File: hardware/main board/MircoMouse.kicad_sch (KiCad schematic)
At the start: 43 parts, among them IC4 W25N01GVZEIG, IC5 LSM6DSLTR, J1 JST-SH 01x06, J2 JST-SH 01x06, J3 JST_XH_B3B, J4 FTSH-107-01-L-DV-K-A, J5 JST-SH 01x06, J6 USB4145-03-0070-C, J7 JST-SH 01x06, U1 LM1117MP-3.3, U2 USBLC6-2SC6

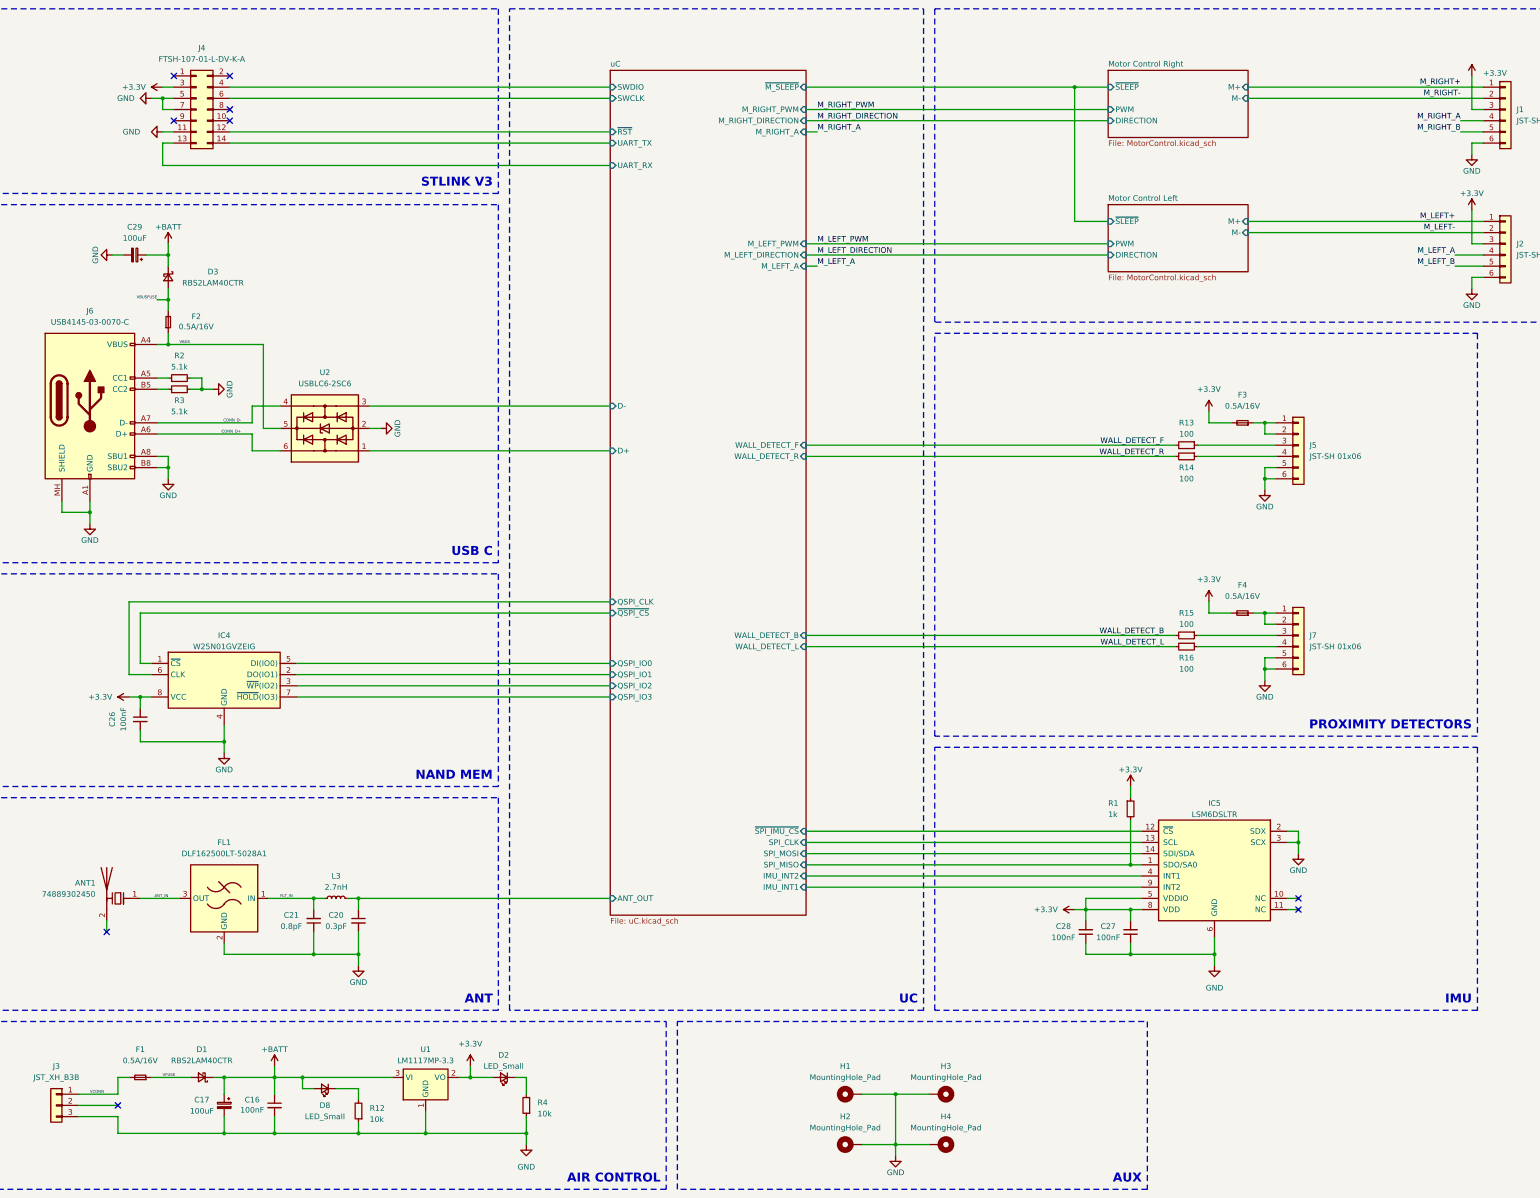
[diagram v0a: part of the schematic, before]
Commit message: final
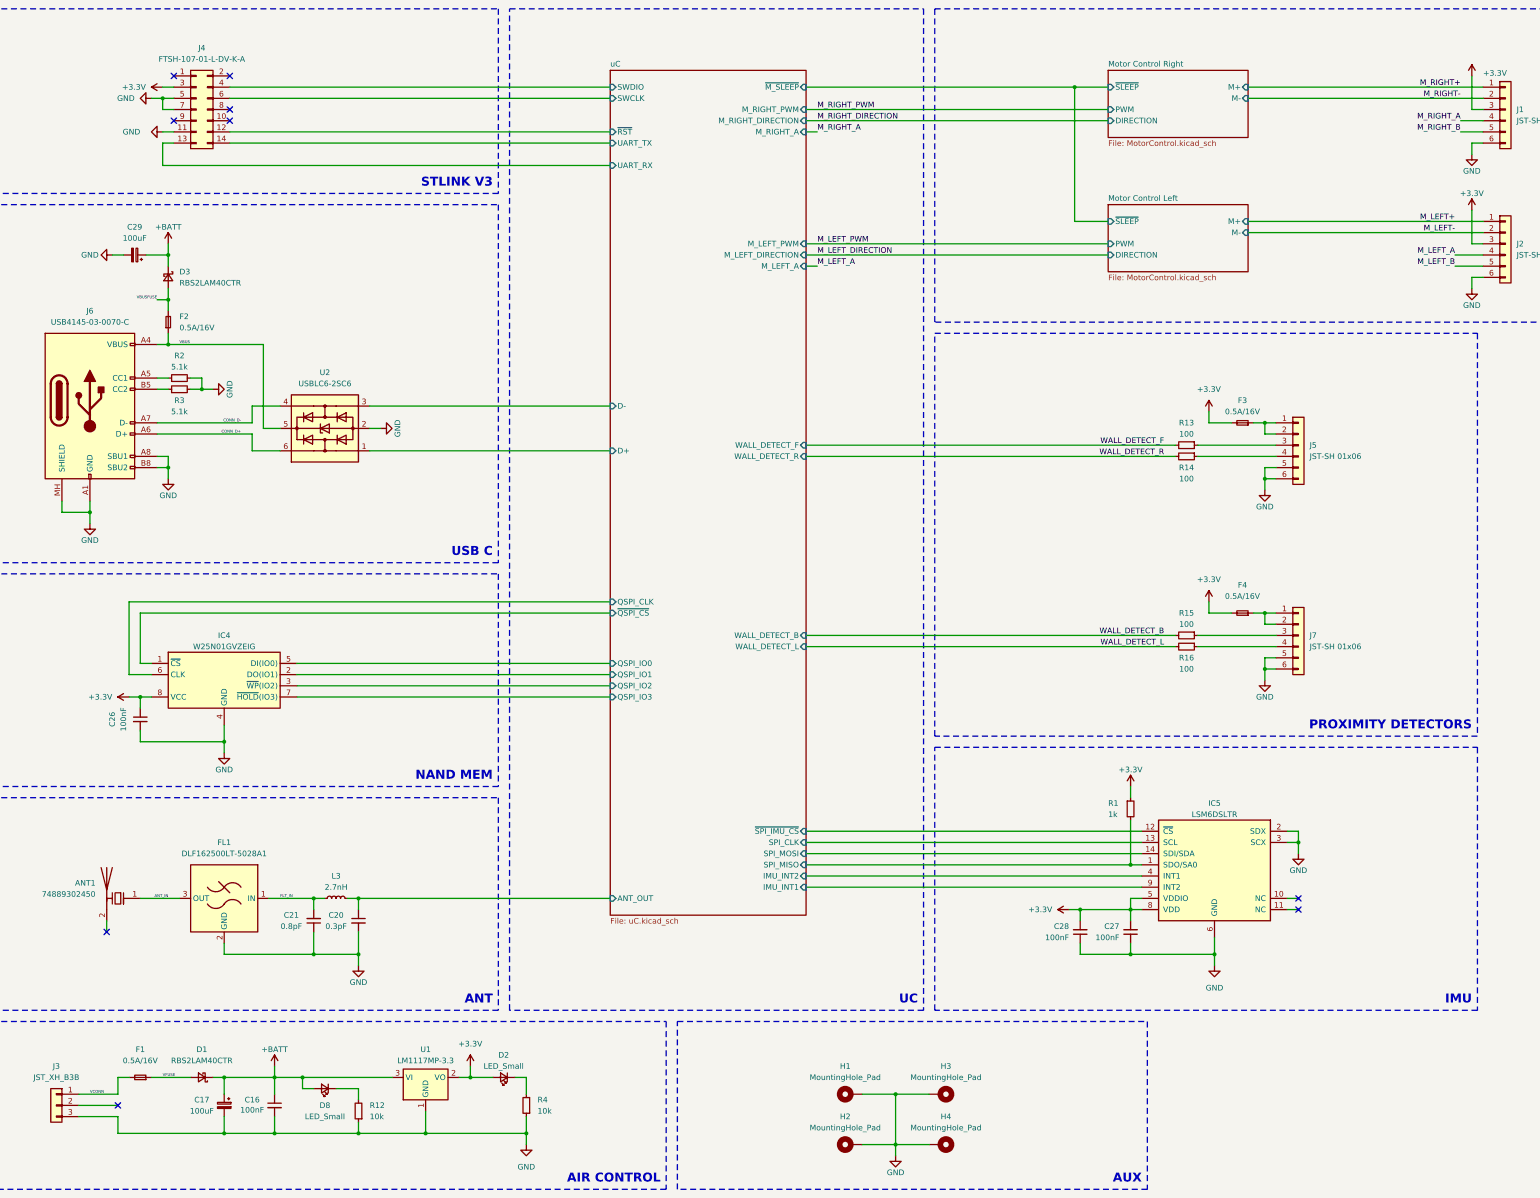
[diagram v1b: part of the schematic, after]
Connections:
- net Motor Control Left/M+ is gone; now on net M_LEFT+: J2.1 (Pin_1)
- net Motor Control Left/M- is gone; now on net M_LEFT-: J2.2 (Pin_2)
- net Motor Control Right/M+ is gone; now on net M_RIGHT+: J1.1 (Pin_1)
- net Motor Control Right/M- is gone; now on net M_RIGHT-: J1.2 (Pin_2)
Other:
- company: (none) -> Made by: Piotr Lesicki
- title: (none) -> Mirco Mouse
- moved on the sheet: C28
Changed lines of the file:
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@@
 	(generator_version "8.0")
 	(paper "A3")
+	(title_block
+		(title "Mirco Mouse")
+		(date "2025-01-02")
+		(rev "1.0")
+		(company "Made by: Piotr Lesicki")
+	)
 	(junction
 		(at 293.37 228.6)
@@
 	)
 	(junction
-		(at 283.21 218.44)
+		(at 74.93 118.11)
 		(diameter 0)
 		(color 0 0 0 0)
 	)
 	(junction
-		(at 74.93 118.11)
+		(at 281.94 218.44)
 		(diameter 0)
 		(color 0 0 0 0)
@@
 	(wire
 		(pts
-			(xy 283.21 226.06) (xy 283.21 228.6)
+			(xy 281.94 226.06) (xy 281.94 228.6)
 		)
 		(stroke
@@
 	(wire
 		(pts
-			(xy 283.21 218.44) (xy 283.21 215.9)
+			(xy 293.37 218.44) (xy 293.37 215.9)
 		)
 		(stroke
@@
 	(wire
 		(pts
-			(xy 283.21 218.44) (xy 280.67 218.44)
+			(xy 281.94 218.44) (xy 279.4 218.44)
 		)
 		(stroke
@@
 	(wire
 		(pts
+			(xy 293.37 218.44) (xy 281.94 218.44)
+		)
+		(stroke
+			(width 0)
+			(type default)
+		)
+	)
+	(wire
+		(pts
 			(xy 219.71 36.83) (xy 288.29 36.83)
 		)
@@
 	(wire
 		(pts
-			(xy 293.37 218.44) (xy 283.21 218.44)
-		)
-		(stroke
-			(width 0)
-			(type default)
-		)
-	)
-	(wire
-		(pts
 			(xy 323.85 107.95) (xy 323.85 110.49)
 		)
@@
 	(wire
 		(pts
-			(xy 295.91 215.9) (xy 283.21 215.9)
+			(xy 295.91 215.9) (xy 293.37 215.9)
 		)
 		(stroke
@@
 	(wire
 		(pts
-			(xy 283.21 220.98) (xy 283.21 218.44)
+			(xy 281.94 220.98) (xy 281.94 218.44)
 		)
 		(stroke
@@
 	(wire
 		(pts
-			(xy 293.37 228.6) (xy 283.21 228.6)
+			(xy 293.37 228.6) (xy 281.94 228.6)
 		)
 		(stroke
@@
 	)
 	(label "M_RIGHT-"
-		(at 368.307 34.1021 180)
+		(at 368.3 34.29 180)
 		(fields_autoplaced yes)
 		(effects
@@
 	)
 	(label "M_RIGHT+"
-		(at 368.307 31.5621 180)
+		(at 368.3 31.75 180)
 		(fields_autoplaced yes)
 		(effects
@@
 	)
 	(label "M_LEFT-"
-		(at 367.0387 64.5351 180)
+		(at 367.03 64.77 180)
 		(fields_autoplaced yes)
 		(effects
@@
 	)
 	(label "M_LEFT+"
-		(at 367.0387 61.9951 180)
+		(at 367.03 62.23 180)
 		(fields_autoplaced yes)
 		(effects
@@
 		(dnp no)
 		(property "Reference" "C27"
-			(at 288.29 222.25 0)
+			(at 290.83 222.25 0)
 			(effects
 				(font
 					(size 1.27 1.27)
 				)
+				(justify left)
 			)
 		)
 		(property "Value" "100nF"
-			(at 288.29 224.79 0)
+			(at 290.83 224.79 0)
 			(effects
 				(font
 					(size 1.27 1.27)
 				)
+				(justify left)
 			)
 		)
@@
 		(dnp no)
 		(property "Reference" "F2"
-			(at 81.28 83.82 90)
+			(at 77.47 83.82 90)
 			(effects
 				(font
 					(size 1.27 1.27)
 				)
+				(justify right)
 			)
 		)
 		(property "Value" "0.5A/16V"
-			(at 81.28 86.1314 90)
+			(at 77.47 86.36 90)
 			(effects
 				(font
 					(size 1.27 1.27)
 				)
+				(justify right)
 			)
 		)
@@
 		)
 		(property "Value" "GND"
-			(at 58.42 69.85 0)
+			(at 57.15 69.85 90)
 			(effects
 				(font
@@
 	(symbol
 		(lib_id "power:+3.3V")
-		(at 280.67 218.44 90)
+		(at 279.4 218.44 90)
 		(mirror x)
 		(unit 1)
@@
 		(dnp no)
 		(property "Reference" "#PWR038"
-			(at 284.48 218.44 0)
+			(at 283.21 218.44 0)
 			(effects
 				(font
@@
 		)
 		(property "Value" "+3.3V"
-			(at 276.86 218.44 90)
+			(at 275.59 218.44 90)
 			(effects
 				(font
@@
 		)
 		(property "Footprint" ""
-			(at 280.67 218.44 0)
+			(at 279.4 218.44 0)
 			(effects
 				(font
@@
 		)
 		(property "Datasheet" ""
-			(at 280.67 218.44 0)
+			(at 279.4 218.44 0)
 			(effects
 				(font
@@
 		)
 		(property "Description" ""
-			(at 280.67 218.44 0)
+			(at 279.4 218.44 0)
 			(effects
 				(font
@@
 		(dnp no)
 		(property "Reference" "D3"
-			(at 85.09 73.66 90)
+			(at 77.47 73.66 90)
 			(effects
 				(font
 					(size 1.27 1.27)
 				)
+				(justify left)
 			)
 		)
 		(property "Value" "RBS2LAM40CTR"
-			(at 85.09 76.2 90)
+			(at 77.47 76.2 90)
 			(effects
 				(font
 					(size 1.27 1.27)
 				)
+				(justify left)
 			)
 		)
@@
 		(on_board yes)
 		(dnp no)
-		(fields_autoplaced yes)
 		(property "Reference" "R12"
-			(at 120.65 263.525 0)
+			(at 120.65 262.89 0)
 			(effects
 				(font
@@
 		)
 		(property "Value" "10k"
-			(at 120.65 266.065 0)
+			(at 120.65 265.43 0)
 			(effects
 				(font
@@
 		(on_board yes)
 		(dnp no)
-		(fields_autoplaced yes)
 		(property "Reference" "R4"
-			(at 158.75 262.255 0)
+			(at 158.75 261.62 0)
 			(effects
 				(font
@@
 		)
 		(property "Value" "10k"
-			(at 158.75 264.795 0)
+			(at 158.75 264.16 0)
 			(effects
 				(font
@@
 	(symbol
 		(lib_id "Device:C_Small")
-		(at 283.21 223.52 180)
+		(at 281.94 223.52 180)
 		(unit 1)
 		(exclude_from_sim no)
@@
 		(dnp no)
 		(property "Reference" "C28"
-			(at 278.13 222.25 0)
+			(at 279.4 222.25 0)
 			(effects
 				(font
 					(size 1.27 1.27)
 				)
+				(justify left)
 			)
 		)
 		(property "Value" "100nF"
-			(at 278.13 224.79 0)
+			(at 279.4 224.79 0)
 			(effects
 				(font
 					(size 1.27 1.27)
 				)
+				(justify left)
 			)
 		)
 		(property "Footprint" "Capacitor_SMD:C_0603_1608Metric"
-			(at 283.21 223.52 0)
+			(at 281.94 223.52 0)
 			(effects
 				(font
@@
 		)
 		(property "Datasheet" "~"
-			(at 283.21 223.52 0)
+			(at 281.94 223.52 0)
 			(effects
 				(font
@@
 		)
 		(property "Description" ""
-			(at 283.21 223.52 0)
+			(at 281.94 223.52 0)
 			(effects
 				(font
@@
 		)
 		(property "Manufacturer_Name" "--"
-			(at 283.21 223.52 0)
+			(at 281.94 223.52 0)
 			(effects
 				(font
@@
 		)
 		(property "Manufacturer_Part_Number" "--"
-			(at 283.21 223.52 0)
+			(at 281.94 223.52 0)
 			(effects
 				(font
@@
 		)
 		(property "Dodane do zamówienia" "20"
-			(at 283.21 223.52 0)
+			(at 281.94 223.52 0)
 			(effects
 				(font
@@
 		)
 		(property "Mouser Part Number" "963-EMK107B7104MA-T"
-			(at 283.21 223.52 0)
+			(at 281.94 223.52 0)
 			(effects
 				(font
@@
 		)
 		(property "Mouser Price/Stock" "https://www.mouser.pl/ProductDetail/TAIYO-YUDEN/EMK107B7104MA-T?qs=I6KAKw0tg2yoDM4kgVF98Q%3D%3D"
-			(at 283.21 223.52 0)
+			(at 281.94 223.52 0)
 			(effects
 				(font
@@
 		(dnp no)
 		(property "Reference" "F3"
-			(at 318.77 101.6 0)
+			(at 318.77 102.87 0)
 			(effects
 				(font
@@
 		)
 		(property "Value" "0.5A/16V"
-			(at 318.77 104.14 0)
+			(at 318.77 105.41 0)
 			(effects
 				(font
